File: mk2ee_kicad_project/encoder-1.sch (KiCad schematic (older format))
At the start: 15 parts, among them J10 Conn_01x02_Male, J8 Conn_02x03_Male, J9 Conn_02x03_Male, U8 AS5047D-ATSM, U9 74HC595

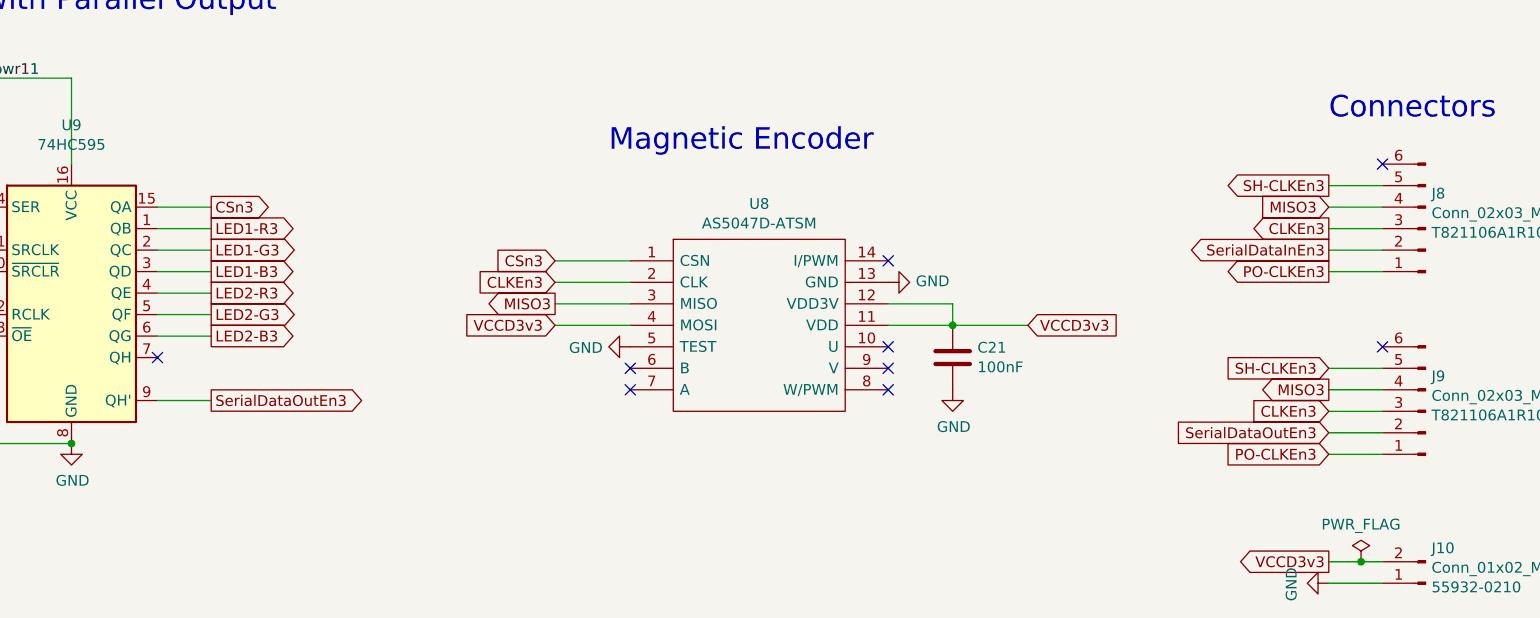
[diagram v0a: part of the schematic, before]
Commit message: all components are connected
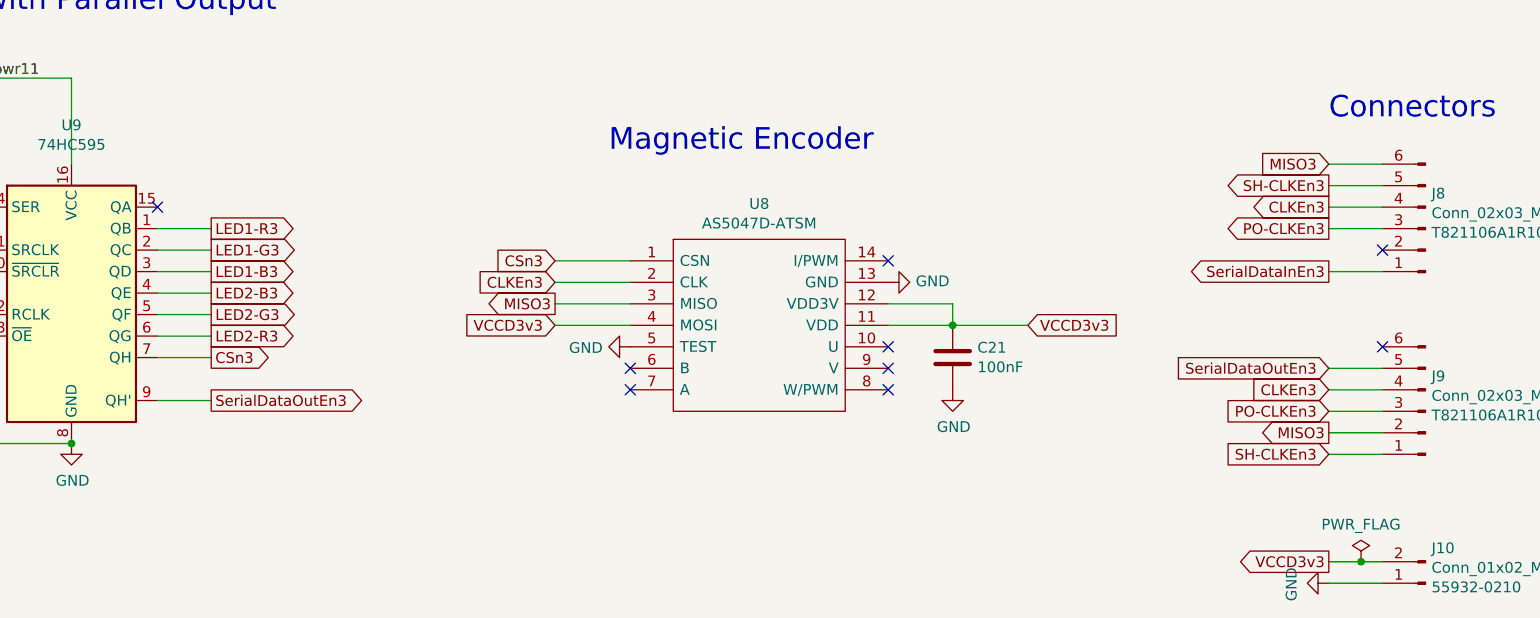
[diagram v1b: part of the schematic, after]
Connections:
- net CLKEn3: now also J8.4 (Pin_4), J9.4 (Pin_4); no longer J8.3 (Pin_3), J9.3 (Pin_3)
- net CSn3: now also U9.7 (QH); no longer U9.15 (QA)
- net LED2-B3: now also U9.4 (QE); no longer U9.6 (QG)
- net LED2-R3: now also U9.6 (QG); no longer U9.4 (QE)
- net MISO3: now also J8.6 (Pin_6), J9.2 (Pin_2); no longer J8.4 (Pin_4), J9.4 (Pin_4)
- net PO-CLKEn3: now also J8.3 (Pin_3), J9.3 (Pin_3); no longer J8.1 (Pin_1), J9.1 (Pin_1)
- net SH-CLKEn3: now also J9.1 (Pin_1); no longer J9.5 (Pin_5)
- net SerialDataInEn3: now also J8.1 (Pin_1); no longer J8.2 (Pin_2)
- net SerialDataOutEn3: now also J9.5 (Pin_5); no longer J9.2 (Pin_2)
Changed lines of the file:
@@
 Comment4 ""
 $EndDescr
-Text GLabel 3950 1900 2    50   Output ~ 0
+Text GLabel 3950 2600 2    50   Output ~ 0
 CSn3
 Text GLabel 3950 2000 2    50   Output ~ 0
@@
 Text GLabel 3950 2200 2    50   Output ~ 0
 LED1-B3
-Text GLabel 3950 2300 2    50   Output ~ 0
+Text GLabel 3950 2500 2    50   Output ~ 0
 LED2-R3
 Text GLabel 3950 2400 2    50   Output ~ 0
 LED2-G3
-NoConn ~ 3700 2600
-Wire Wire Line
-	3700 1900 3950 1900
+Wire Wire Line
+	3700 2600 3950 2600
 Wire Wire Line
 	3700 2000 3950 2000
@@
 	3700 2200 3950 2200
 Wire Wire Line
-	3700 2300 3950 2300
+	3700 2500 3950 2500
 Wire Wire Line
 	3700 2400 3950 2400
-Text GLabel 9150 2000 0    50   Output ~ 0
+Text GLabel 9150 1900 0    50   Output ~ 0
 CLKEn3
-Text GLabel 9150 1900 0    50   Input ~ 0
+Text GLabel 9150 1700 0    50   Input ~ 0
 MISO3
 Text GLabel 9150 1800 0    50   Output ~ 0
 SH-CLKEn3
-Text GLabel 9150 2100 0    50   Output ~ 0
+Text GLabel 9150 2200 0    50   Output ~ 0
 SerialDataInEn3
-Text GLabel 9150 2200 0    50   Output ~ 0
+Text GLabel 9150 2000 0    50   Output ~ 0
 PO-CLKEn3
 Wire Wire Line
 	9150 1800 9400 1800
 Wire Wire Line
+	9150 1700 9400 1700
+Wire Wire Line
 	9150 1900 9400 1900
 Wire Wire Line
+	9150 2200 9400 2200
+Wire Wire Line
 	9150 2000 9400 2000
 Wire Wire Line
-	9150 2100 9400 2100
-Wire Wire Line
-	9150 2200 9400 2200
+	9150 3050 9400 3050
+Wire Wire Line
+	9150 2950 9400 2950
+Wire Wire Line
+	9150 2750 9400 2750
 Wire Wire Line
 	9150 2650 9400 2650
 Wire Wire Line
-	9150 2750 9400 2750
-Wire Wire Line
 	9150 2850 9400 2850
-Wire Wire Line
-	9150 2950 9400 2950
-Wire Wire Line
-	9150 3050 9400 3050
 Text GLabel 2250 1300 0    50   Input ~ 0
 VCCD3v3
@@
 Wire Wire Line
 	2650 1900 2900 1900
-Text GLabel 3950 2500 2    50   Output ~ 0
+Text GLabel 3950 2300 2    50   Output ~ 0
 LED2-B3
 Wire Wire Line
-	3700 2500 3950 2500
+	3700 2300 3950 2300
+Text GLabel 9150 2750 0    50   Input ~ 0
+CLKEn3
+Text GLabel 9150 2950 0    50   Output ~ 0
+MISO3
+Text GLabel 9150 3050 0    50   Input ~ 0
+SH-CLKEn3
+Text GLabel 9150 2650 0    50   Input ~ 0
+SerialDataOutEn3
 Text GLabel 9150 2850 0    50   Input ~ 0
-CLKEn3
-Text GLabel 9150 2750 0    50   Output ~ 0
-MISO3
-Text GLabel 9150 2650 0    50   Input ~ 0
-SH-CLKEn3
-Text GLabel 9150 2950 0    50   Input ~ 0
-SerialDataOutEn3
-Text GLabel 9150 3050 0    50   Input ~ 0
 PO-CLKEn3
 $Comp
@@
 	-1   0    0    1
 $EndComp
-NoConn ~ 9400 2550
-NoConn ~ 9400 1700
 $Comp
 L Connector:Conn_01x02_Male J?
@@
 Wire Wire Line
 	2450 1300 2750 1300
+NoConn ~ 3700 1900
+NoConn ~ 9400 2100
+NoConn ~ 9400 2550
 $EndSCHEMATC
